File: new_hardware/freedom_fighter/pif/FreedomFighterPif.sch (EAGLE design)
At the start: 47 parts, among them U1 PIA6821, U10 74LS74D, U11 74LS138D, U12 74LS125D, U2 HM6116P-A, U4 HD68A09EP, U6 74LS245DW, U7 74LS10D, U9 74LS04D

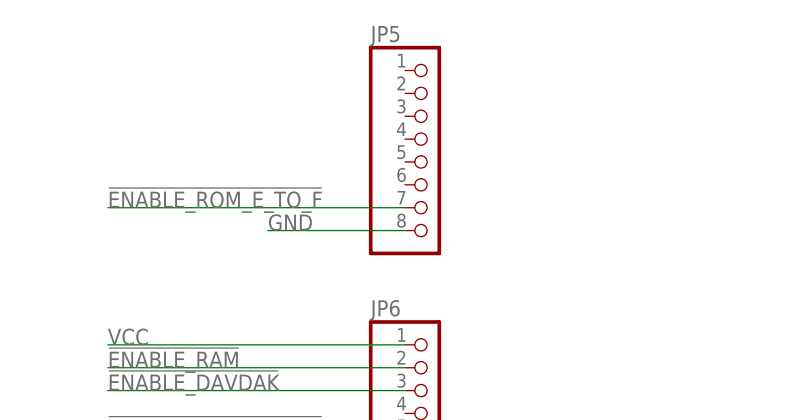
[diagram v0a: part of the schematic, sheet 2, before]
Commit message: 3/4 of the way finished, about to add ground plane
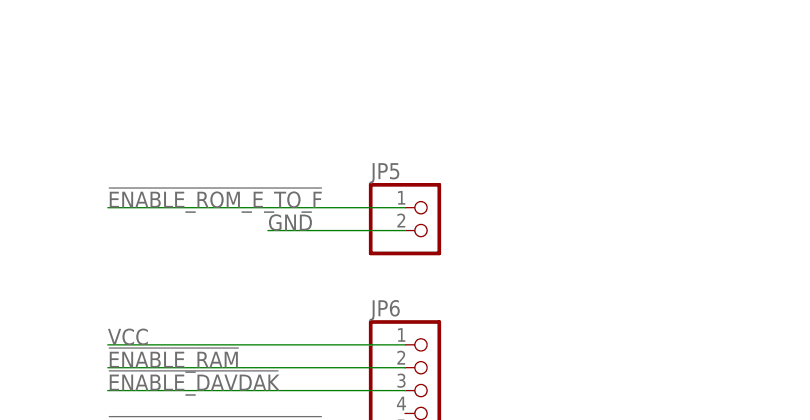
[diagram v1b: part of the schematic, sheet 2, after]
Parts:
- JP5: device pinhead:PINHD-1X8 -> pinhead:PINHD-1X2
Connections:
- net !ENABLE_ROM_E_TO_F: now also JP5.1; no longer JP5.7
- net GND: now also JP5.2; no longer JP5.8
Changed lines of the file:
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@@
 <part name="JP1" library="pinhead" deviceset="PINHD-1X20" device=""/>
 <part name="JP4" library="pinhead" deviceset="PINHD-1X20" device=""/>
-<part name="JP5" library="pinhead" deviceset="PINHD-1X8" device=""/>
 <part name="JP6" library="pinhead" deviceset="PINHD-1X8" device=""/>
 <part name="JP7" library="pinhead" deviceset="PINHD-1X7" device=""/>
@@
 <part name="L1" library="SparkFun" deviceset="INDUCTOR" device="H*" technology="1206" value="2.2uH"/>
 <part name="R100" library="SparkFun" deviceset="RESISTOR" device="1206" value="680"/>
+<part name="JP5" library="pinhead" deviceset="PINHD-1X2" device=""/>
 </parts>
 <sheets>
@@
 <instance part="JP1" gate="A" x="73.66" y="96.52"/>
 <instance part="JP4" gate="A" x="101.6" y="96.52"/>
-<instance part="JP5" gate="A" x="154.94" y="109.22"/>
 <instance part="JP6" gate="A" x="154.94" y="78.74"/>
 <instance part="JP7" gate="A" x="236.22" y="111.76"/>
 <instance part="JP8" gate="A" x="236.22" y="83.82"/>
+<instance part="JP5" gate="G$1" x="154.94" y="101.6"/>
 </instances>
 <busses>
@@
 </segment>
 <segment>
-<pinref part="JP5" gate="A" pin="8"/>
 <wire x1="152.4" y1="101.6" x2="137.16" y2="101.6" width="0.1524" layer="91"/>
 <label x="137.16" y="101.6" size="1.778" layer="95"/>
+<pinref part="JP5" gate="G$1" pin="2"/>
 </segment>
 <segment>
@@
 <net name="!ENABLE_ROM_E_TO_F" class="0">
 <segment>
-<pinref part="JP5" gate="A" pin="7"/>
 <wire x1="152.4" y1="104.14" x2="119.38" y2="104.14" width="0.1524" layer="91"/>
 <label x="119.38" y="104.14" size="1.778" layer="95"/>
-</segment>
-</net>
+<pinref part="JP5" gate="G$1" pin="1"/>
+</segment>
+</net>
